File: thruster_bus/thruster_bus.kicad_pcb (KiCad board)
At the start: 2 copper layers, 30.5 x 36.8 mm, 9 parts, among them P1 CONN_01X03, P2 CONN_01X03, P3 CONN_01X03, P4 CONN_01X06, P5 CONN_01X03

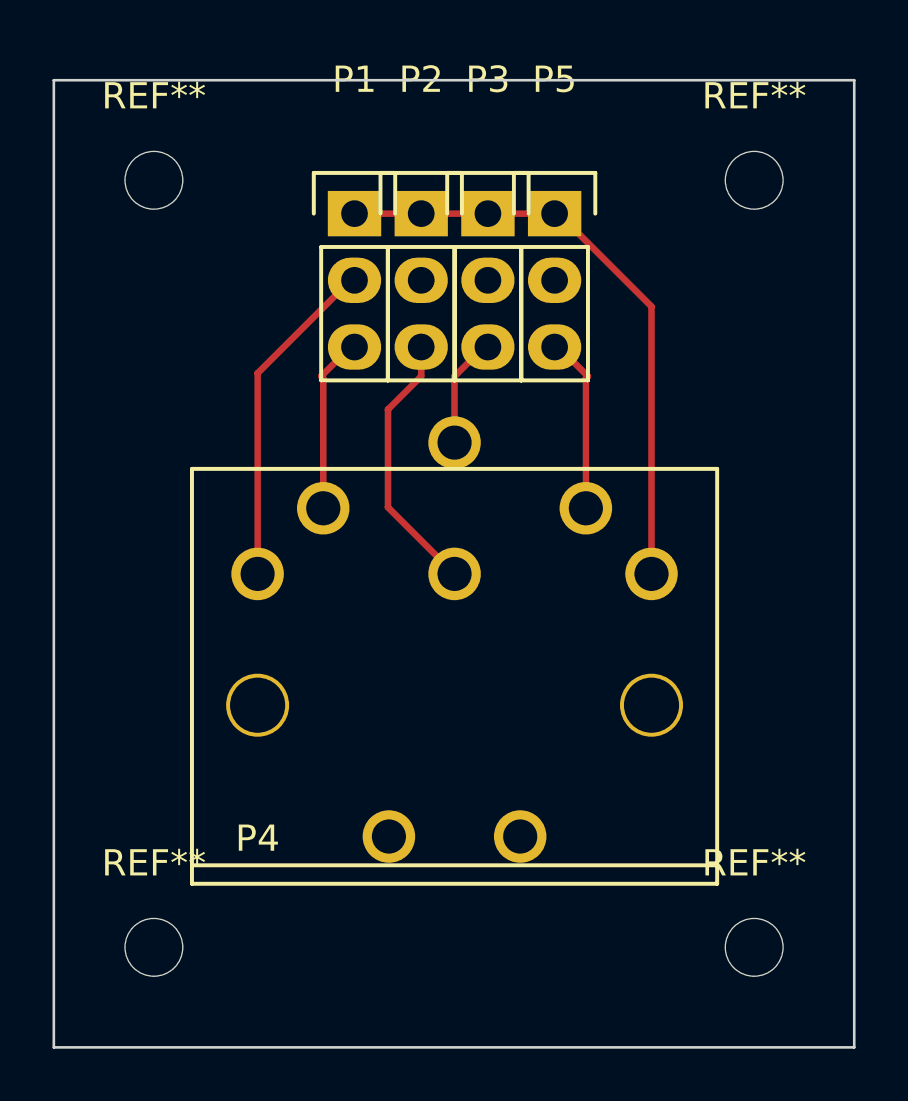
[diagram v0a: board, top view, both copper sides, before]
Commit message: Addition of labels for OSH Park printing
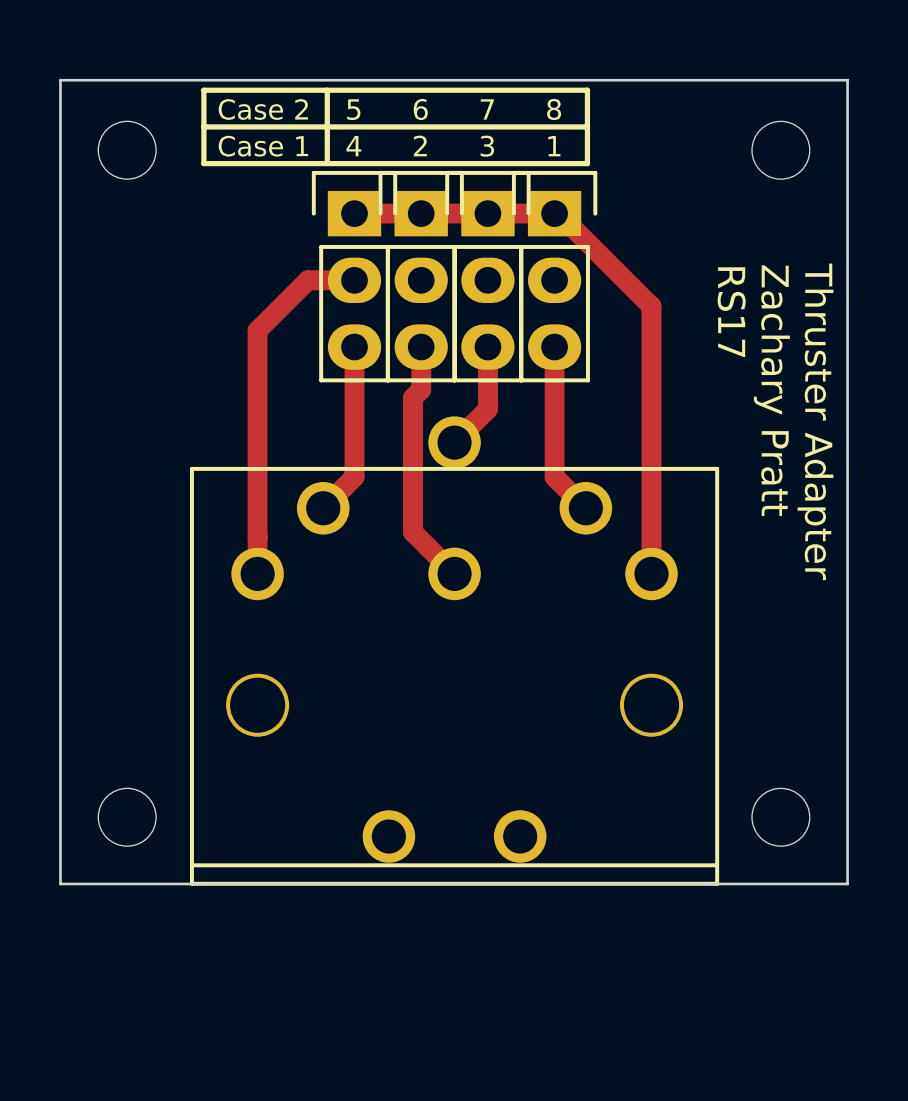
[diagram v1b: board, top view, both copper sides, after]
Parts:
- moved REF** 5.06 mm to (145.0, 104.3)
- moved REF** 5.06 mm to (169.9, 104.3)
- moved REF** 1.53 mm to (145.0, 78.9)
- moved REF** 1.53 mm to (169.9, 78.9)
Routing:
- net (no net): track 30.5 -> 0.00 mm
- net /ESC5V: track 12.8 -> 13.7 mm
- net /2: track 10.2 -> 9.42 mm
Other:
- board size 30.5 x 36.8 mm -> 30 x 30.6 mm
- net class Default: trace_width 0.25 -> 0.758
- board text added: "1"
- board text added: "2"
- board text added: "3"
- board text added: "4"
- board text added: "5"
- board text added: "6"
- board text added: "7"
- board text added: "8"
- board text added: "Case 1"
- board text added: "Case 2"
- board text added: "Thruster Adapter Zachary Pratt RS17"
